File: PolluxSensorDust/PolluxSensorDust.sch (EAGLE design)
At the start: 5 parts

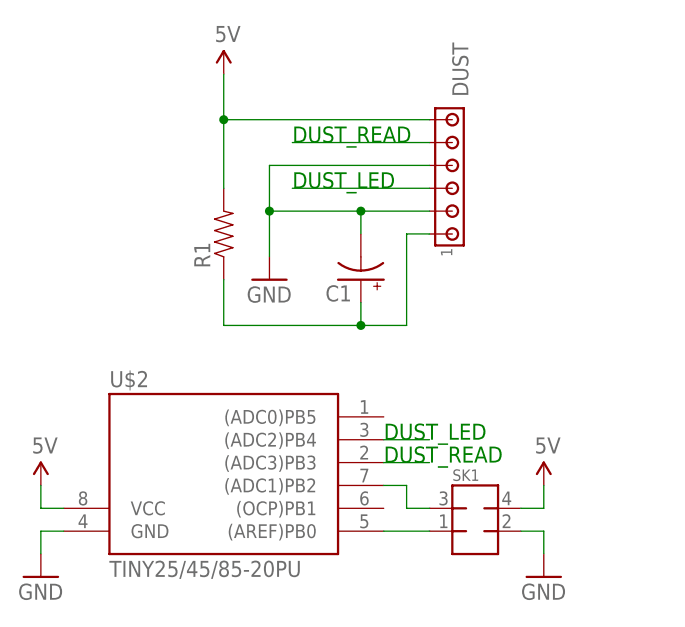
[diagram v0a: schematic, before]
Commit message: improve sensor board
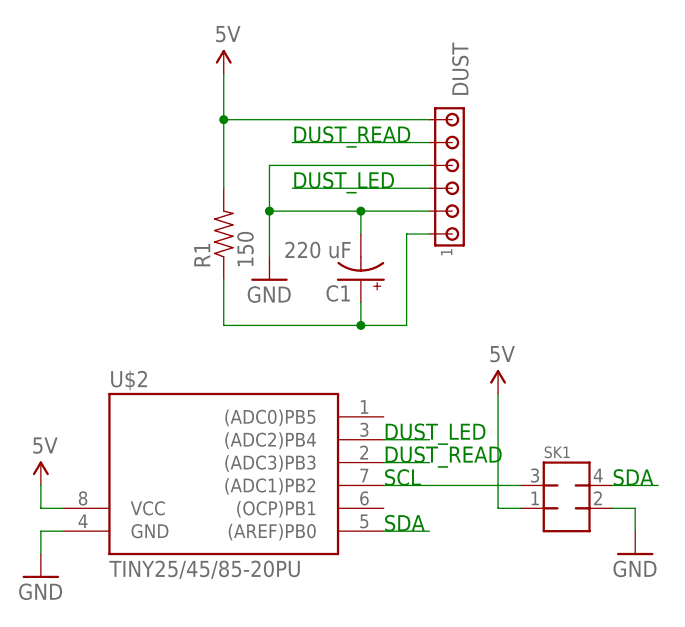
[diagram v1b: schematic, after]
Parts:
- C1: value (none) -> 220 uF
- R1: value (none) -> 150
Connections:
- removed net N$2: SK1.1, U$2.(AREF)PB0
- new net SDA: SK1.4, U$2.(AREF)PB0
- net 5V: now also SK1.1; no longer SK1.4
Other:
- note added: "SCL"
- note added: "SDA"
- moved on the sheet: SK1
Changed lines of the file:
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@@
 <part name="SK1" library="jt-con-micromatch" deviceset="MMATCH-8-*" device="PTH"/>
 <part name="U$2" library="avr-7" deviceset="TINY25/45/85" device="-20PU"/>
-<part name="C1" library="SparkFun" deviceset="CAP_POL" device="PTH4"/>
-<part name="R1" library="SparkFun" deviceset="RESISTOR" device="AXIAL-0.3"/>
+<part name="C1" library="SparkFun" deviceset="CAP_POL" device="PTH4" value="220 uF"/>
+<part name="R1" library="SparkFun" deviceset="RESISTOR" device="AXIAL-0.3" value="150"/>
 <part name="DUST" library="con-amp" deviceset="MTA06-100" device=""/>
 <part name="U$3" library="SparkFun" deviceset="5V" device=""/>
@@
 <text x="60.96" y="60.96" size="1.778" layer="91">DUST_LED</text>
 <text x="60.96" y="66.04" size="1.778" layer="91">DUST_READ</text>
+<text x="71.12" y="27.94" size="1.778" layer="91">SCL</text>
+<text x="71.12" y="22.86" size="1.778" layer="91">SDA</text>
+<text x="96.52" y="27.94" size="1.778" layer="91">SDA</text>
 </plain>
 <instances>
 <instance part="U$1" gate="G$1" x="53.34" y="73.66"/>
-<instance part="GND1" gate="1" x="88.9" y="17.78"/>
-<instance part="SK1" gate="G$1" x="81.28" y="22.86"/>
+<instance part="GND1" gate="1" x="99.06" y="20.32"/>
+<instance part="SK1" gate="G$1" x="91.44" y="25.4"/>
 <instance part="U$2" gate="G$1" x="53.34" y="27.94"/>
 <instance part="C1" gate="G$1" x="68.58" y="50.8" rot="R180"/>
@@
 <instance part="DUST" gate="G$1" x="78.74" y="60.96" rot="MR90"/>
 <instance part="U$3" gate="G$1" x="33.02" y="27.94"/>
-<instance part="U$4" gate="G$1" x="88.9" y="27.94"/>
+<instance part="U$4" gate="G$1" x="83.82" y="38.1"/>
 <instance part="GND2" gate="1" x="33.02" y="17.78"/>
 <instance part="GND3" gate="1" x="58.42" y="50.8"/>
@@
 </busses>
 <nets>
-<net name="N$2" class="0">
-<segment>
-<pinref part="SK1" gate="G$1" pin="1"/>
-<pinref part="U$2" gate="G$1" pin="(AREF)PB0"/>
-<wire x1="76.2" y1="22.86" x2="71.12" y2="22.86" width="0.1524" layer="91"/>
-</segment>
-</net>
 <net name="5V" class="0">
-<segment>
-<pinref part="SK1" gate="G$1" pin="4"/>
-<wire x1="86.36" y1="25.4" x2="88.9" y2="25.4" width="0.1524" layer="91"/>
-<pinref part="U$4" gate="G$1" pin="5V"/>
-<wire x1="88.9" y1="25.4" x2="88.9" y2="27.94" width="0.1524" layer="91"/>
-</segment>
 <segment>
 <pinref part="U$2" gate="G$1" pin="VCC"/>
@@
 <pinref part="DUST" gate="G$1" pin="6"/>
 <junction x="53.34" y="68.58"/>
+</segment>
+<segment>
+<pinref part="SK1" gate="G$1" pin="1"/>
+<wire x1="86.36" y1="25.4" x2="83.82" y2="25.4" width="0.1524" layer="91"/>
+<wire x1="83.82" y1="25.4" x2="83.82" y2="38.1" width="0.1524" layer="91"/>
+<pinref part="U$4" gate="G$1" pin="5V"/>
 </segment>
 </net>
@@
 </segment>
 <segment>
-<pinref part="SK1" gate="G$1" pin="2"/>
-<wire x1="86.36" y1="22.86" x2="88.9" y2="22.86" width="0.1524" layer="91"/>
-<pinref part="GND1" gate="1" pin="GND"/>
-<wire x1="88.9" y1="22.86" x2="88.9" y2="20.32" width="0.1524" layer="91"/>
-</segment>
-<segment>
 <pinref part="GND3" gate="1" pin="GND"/>
 <wire x1="58.42" y1="53.34" x2="58.42" y2="58.42" width="0.1524" layer="91"/>
@@
 <junction x="68.58" y="58.42"/>
 </segment>
-</net>
-<net name="N$1" class="0">
 <segment>
-<pinref part="U$2" gate="G$1" pin="(ADC1)PB2"/>
-<wire x1="71.12" y1="27.94" x2="73.66" y2="27.94" width="0.1524" layer="91"/>
-<wire x1="73.66" y1="27.94" x2="73.66" y2="25.4" width="0.1524" layer="91"/>
-<pinref part="SK1" gate="G$1" pin="3"/>
-<wire x1="73.66" y1="25.4" x2="76.2" y2="25.4" width="0.1524" layer="91"/>
+<pinref part="SK1" gate="G$1" pin="2"/>
+<pinref part="GND1" gate="1" pin="GND"/>
+<wire x1="96.52" y1="25.4" x2="99.06" y2="25.4" width="0.1524" layer="91"/>
+<wire x1="99.06" y1="25.4" x2="99.06" y2="22.86" width="0.1524" layer="91"/>
 </segment>
 </net>
@@
 </segment>
 </net>
+<net name="N$1" class="0">
+<segment>
+<pinref part="U$2" gate="G$1" pin="(ADC1)PB2"/>
+<pinref part="SK1" gate="G$1" pin="3"/>
+<wire x1="71.12" y1="27.94" x2="86.36" y2="27.94" width="0.1524" layer="91"/>
+</segment>
+</net>
+<net name="SDA" class="0">
+<segment>
+<pinref part="U$2" gate="G$1" pin="(AREF)PB0"/>
+<wire x1="71.12" y1="22.86" x2="76.2" y2="22.86" width="0.1524" layer="91"/>
+</segment>
+<segment>
+<pinref part="SK1" gate="G$1" pin="4"/>
+<wire x1="96.52" y1="27.94" x2="101.6" y2="27.94" width="0.1524" layer="91"/>
+</segment>
+</net>
